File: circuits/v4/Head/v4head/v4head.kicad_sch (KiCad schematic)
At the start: 19 parts, among them J1 Raspberry_Pi_2_3

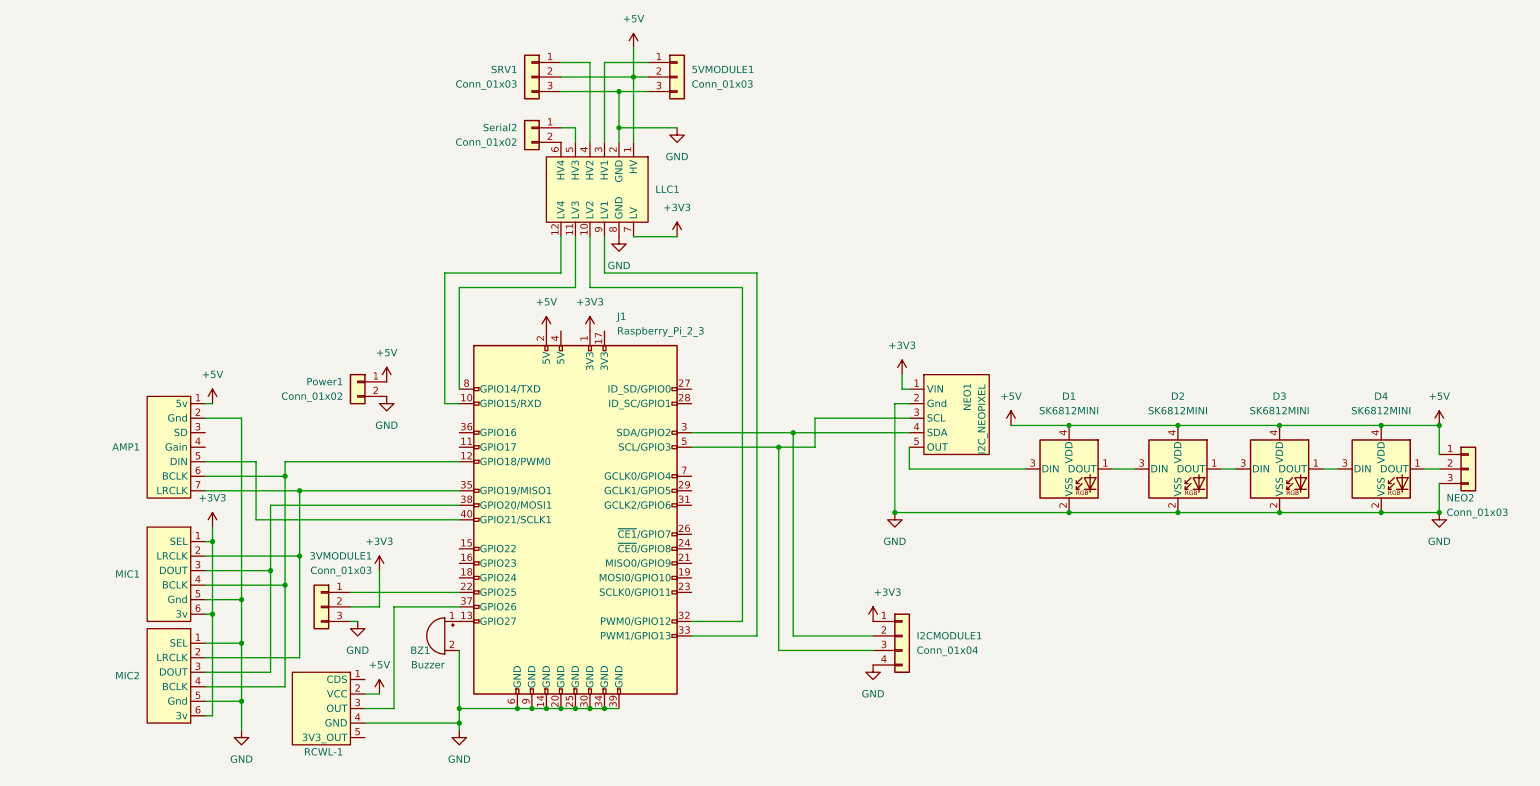
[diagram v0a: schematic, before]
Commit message: Updates to circuit
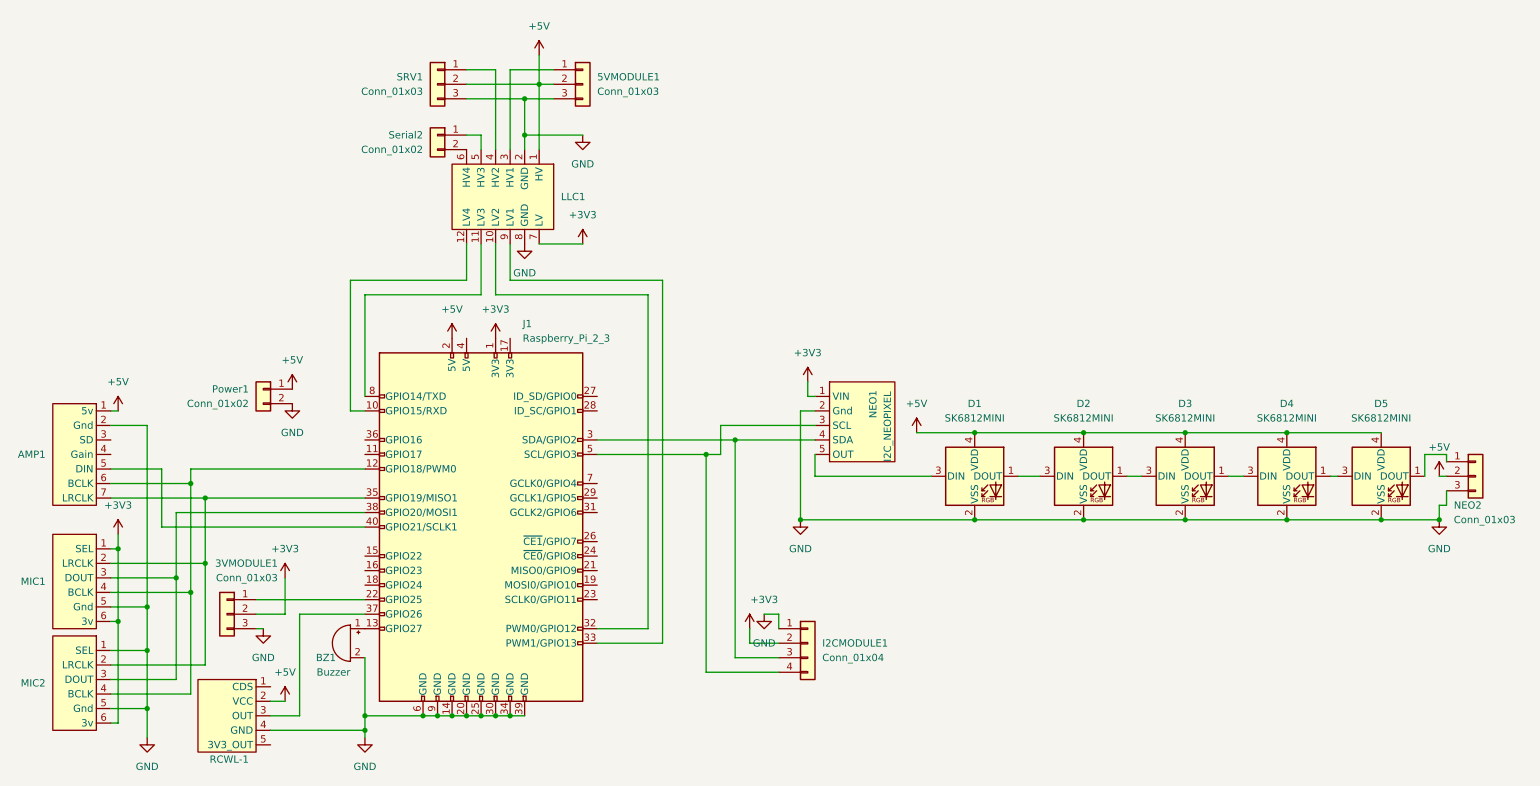
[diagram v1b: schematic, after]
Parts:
- added D5: SK6812MINI, LED_SMD:LED_SK6812MINI_PLCC4_3.5x3.5mm_P1.75mm, symbol LED:SK6812MINI
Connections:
- net +3V3: now also I2CMODULE1.2 (Pin_2); no longer I2CMODULE1.1 (Pin_1)
- net +5V: now also NEO2.2 (Pin_2), D5.4 (VDD); no longer NEO2.1 (Pin_1)
- net GND: now also I2CMODULE1.1 (Pin_1), D5.2 (VSS); no longer I2CMODULE1.4 (Pin_4)
- net at D4.1 (DOUT): now also D5.3 (DIN); no longer NEO2.2 (Pin_2)
- net at J1.3 (SDA/GPIO2), NEO1.4 (SDA): now also I2CMODULE1.3 (Pin_3); no longer I2CMODULE1.2 (Pin_2)
- net at J1.5 (SCL/GPIO3), NEO1.3 (SCL): now also I2CMODULE1.4 (Pin_4); no longer I2CMODULE1.3 (Pin_3)
- new net: D5.1 (DOUT), NEO2.1 (Pin_1)
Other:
- moved on the sheet: 3VMODULE1, 5VMODULE1, AMP1, BZ1, D1, D2, D3, D4, I2CMODULE1, J1, LLC1, MIC1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
